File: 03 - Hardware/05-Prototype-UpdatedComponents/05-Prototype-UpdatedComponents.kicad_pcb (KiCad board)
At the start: 2 copper layers, 83.7 x 70.6 mm, 32 parts, among them J0 Barrel_Jack, J1 Conn_01x03_Male, J2 Conn_01x03_Male, J3 4P4C, J4 4P4C, J5 Conn_01x03_Male, U0 YAAJ_BluePill, U1 LM317_TO-220, U2 LM317_TO-220, U3 microSD_Module_3V3_Horizontal, U4 DS3231_Module_FullAccess, U5 SX1278_Minimal, U6 MCP6002-xP, U7 BME280_I2C_New_LK888

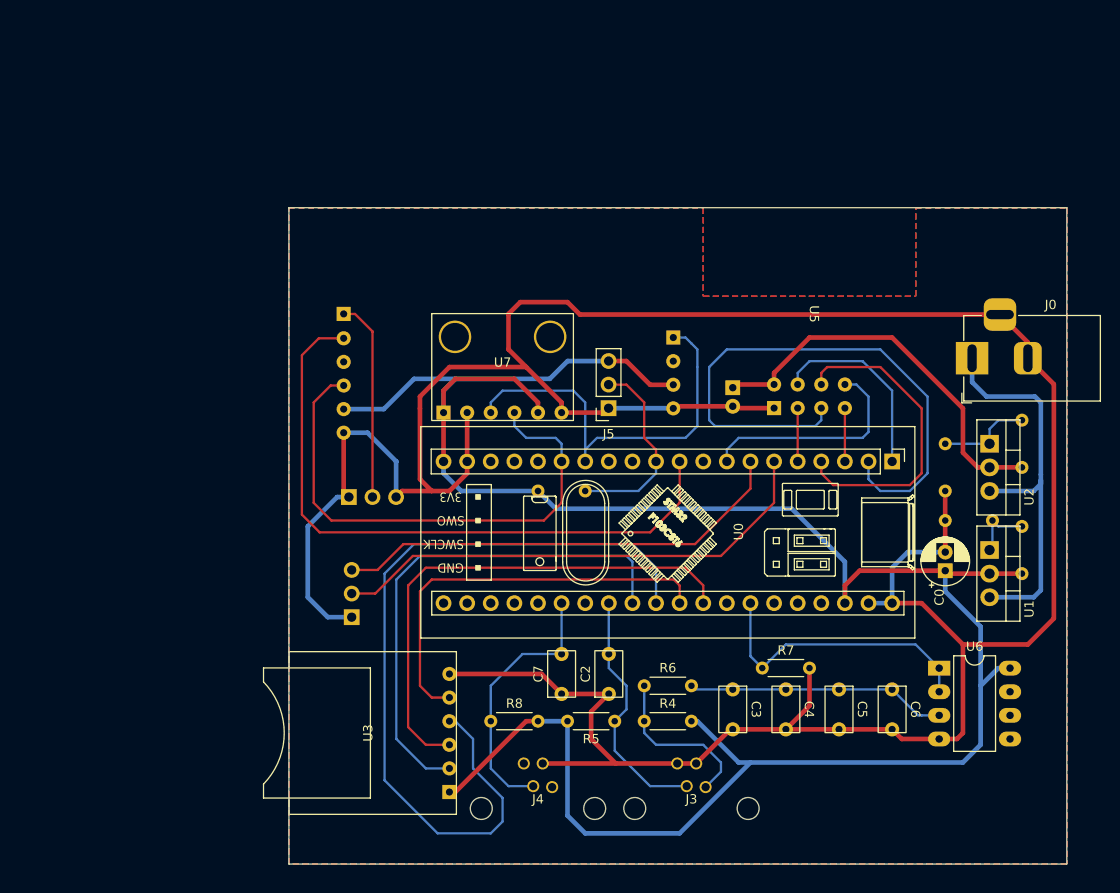
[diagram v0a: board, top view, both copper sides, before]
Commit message: Finalise 2nd version
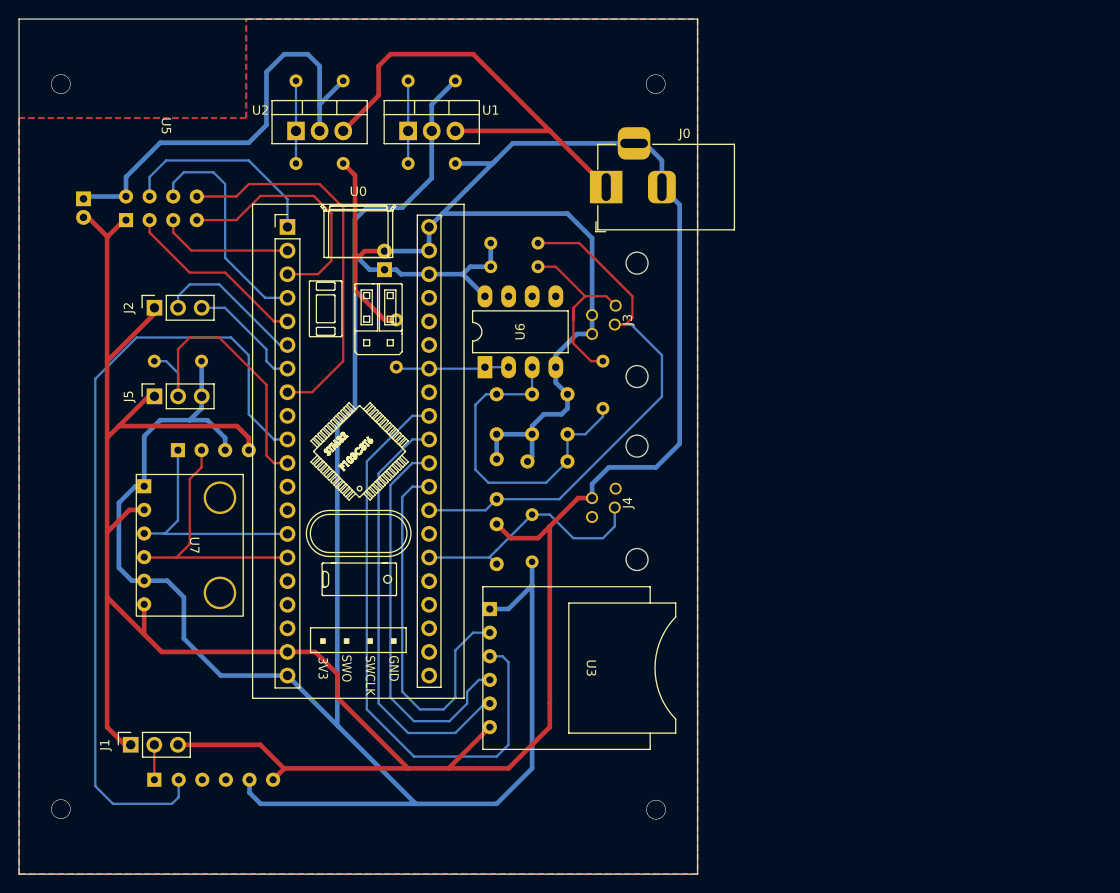
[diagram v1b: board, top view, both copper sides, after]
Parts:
- C0, C2, C3, C4, C5, C6, C7, R4, R5, R6, R7, R8: moved to B.Cu
- J1, J2: moved to F.Cu
- U1, U2: value LM317_TO-220 -> LM317
- U3: value microSD_Module_3V3_Horizontal -> microSD_Module
- U4: value DS3231_Module_FullAccess -> DS3231
- U5: value SX1278_Minimal -> SX1278
- U7: value BME280_I2C_New_LK888 -> BME280
- moved R2 84.0 mm to (142.9, 60.6), turned to 180 degrees
- moved U2 81.9 mm to (137.8, 66.0), turned to 0 degrees
- moved R0 80.8 mm to (154.9, 60.6), turned to 180 degrees
- moved U1 77.1 mm to (149.9, 66.0), turned to 0 degrees
- moved R3 76.1 mm to (137.8, 69.5), turned to 0 degrees
- moved R1 73.7 mm to (149.9, 69.5), turned to 0 degrees
- moved C1 72.7 mm to (114.9, 73.3)
- moved U5 72.6 mm to (123.3, 65.5)
- moved U0 69.8 mm to (136.9, 76.4), turned to 0 degrees
- moved C0 68.5 mm to (147.3, 81.0)
- moved U6 58.6 mm to (158.1, 91.5), turned to 90 degrees
- moved R7 58.1 mm to (148.6, 86.4), turned to -90 degrees
- moved R4 53.4 mm to (158.8, 80.6), turned to 0 degrees
- moved J3 52.5 mm to (174.0, 86.4), turned to 90 degrees
- moved R5 52.1 mm to (158.8, 78.1)
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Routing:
- net GND: track 332.8 -> 390.5 mm
- net LoRa_SCLK: track 63.8 -> 14.4 mm
- net SPI1_SCK: track 86.7 -> 42.3 mm
- net UART_TX: track 53.9 -> 16.3 mm
- net UART_RX: track 49.4 -> 12.7 mm
- net Anemometer: track 26.5 -> 58.0 mm
- net I2C_SDA: track 56.7 -> 28.2 mm
- net LoRa_MISO: track 5.74 -> 26.7 mm
- net WindVane_filtered: track 31.2 -> 12.2 mm
- net I2C_CLK: track 43.1 -> 25.1 mm
- net /32768Hz out: track 21.7 -> 3.76 mm
- net LoRa_DIO0: track 24.2 -> 41.2 mm
- net RTC_ALARM: track 69.6 -> 86.5 mm
- net MICROSD_NCSS: track 55.3 -> 40.9 mm
- net LoRa_Reset: track 5.74 -> 20.1 mm
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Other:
- board size 83.7 x 70.6 mm -> 73 x 92 mm
